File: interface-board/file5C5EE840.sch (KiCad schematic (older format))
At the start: 16 parts, among them Q1 Q_NMOS_GDS, Q2 Q_NMOS_GDS, Q3 Q_NMOS_GDS, Q4 Q_NMOS_GDS

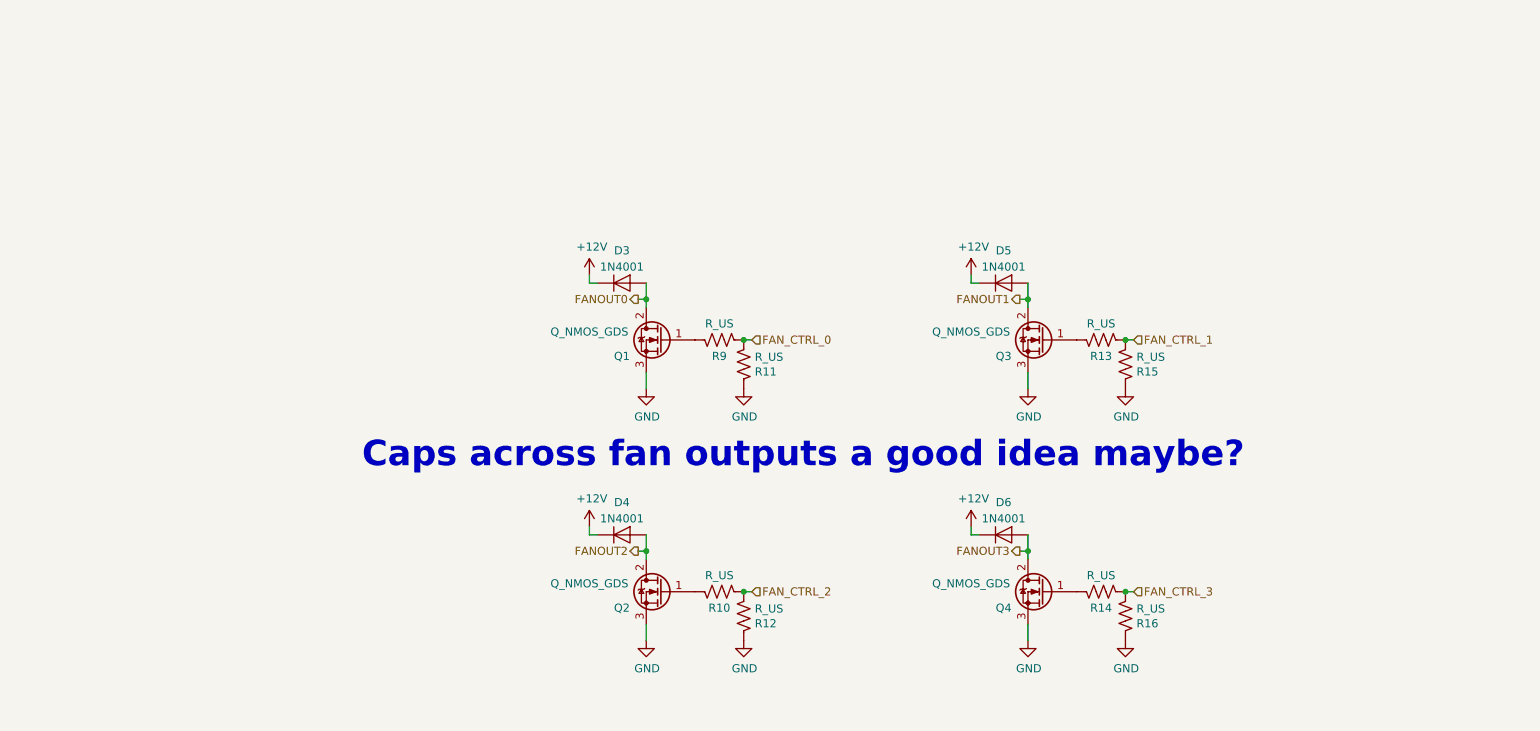
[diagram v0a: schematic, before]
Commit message: Getting there with layout of big board...
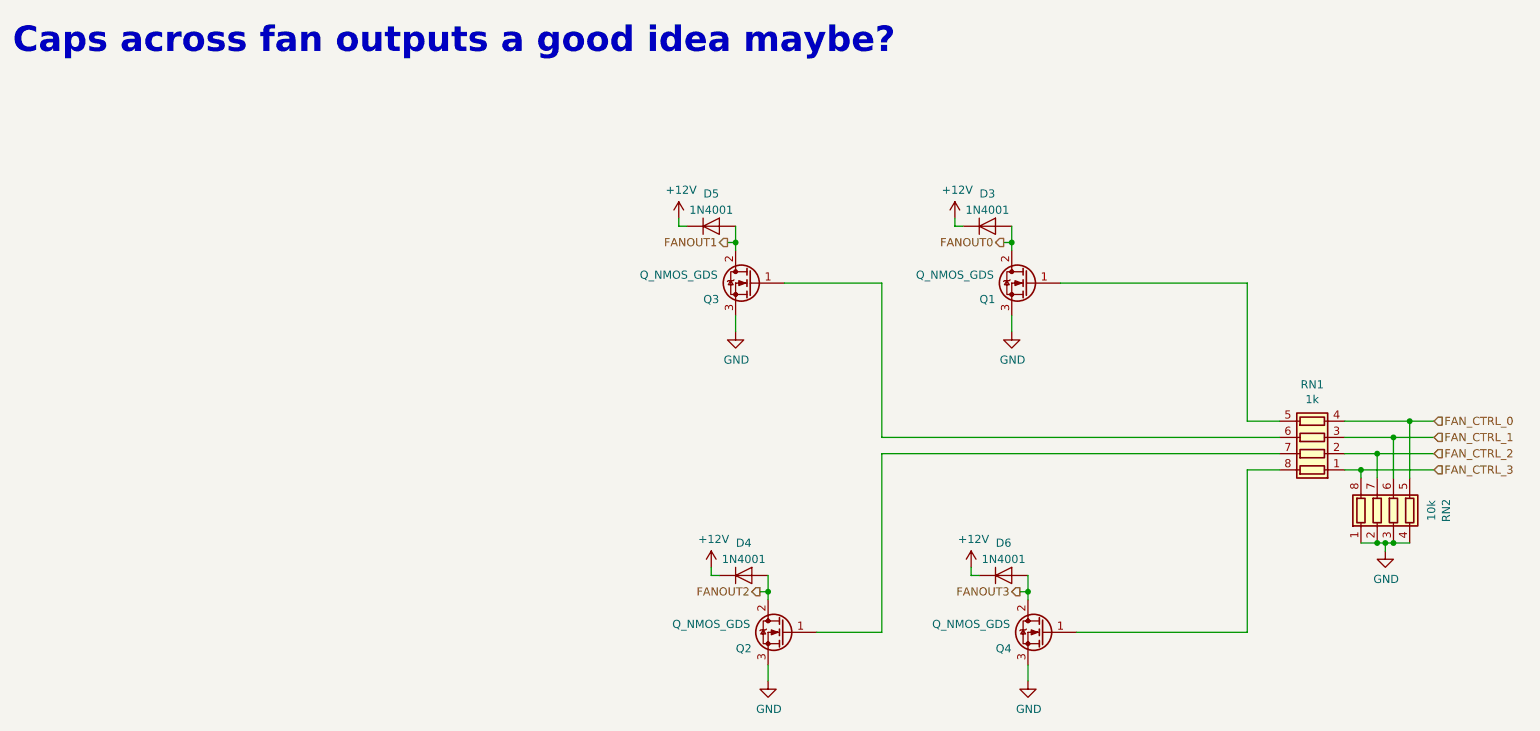
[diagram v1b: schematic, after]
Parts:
- removed R10, R11, R12, R13, R14, R15, R16, R9: R_US, Resistor_SMD:R_0603_1608Metric, symbol Device:R_US
- added RN1: 1k, Resistor_SMD:R_Array_Convex_4x0603, symbol Device:R_Pack04
- added RN2: 10k, Resistor_SMD:R_Array_Convex_4x0603, symbol Device:R_Pack04
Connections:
- net FAN_CTRL_0: now also RN1.4 (R4.1), RN2.5 (R4.2)
- net FAN_CTRL_1: now also RN1.3 (R3.1), RN2.6 (R3.2)
- net FAN_CTRL_2: now also RN1.2 (R2.1), RN2.7 (R2.2)
- net FAN_CTRL_3: now also RN1.1 (R1.1), RN2.8 (R1.2)
- net GND: now also RN2.1 (R1.1), RN2.2 (R2.1), RN2.3 (R3.1), RN2.4 (R4.1)
- net at Q1.1 (G): now also RN1.5 (R4.2)
- net at Q3.1 (G): now also RN1.6 (R3.2)
- net at Q2.1 (G): now also RN1.7 (R2.2)
- net at Q4.1 (G): now also RN1.8 (R1.2)
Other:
- moved on the sheet: D3, D4, D5, D6, Q1, Q2, Q3, Q4
